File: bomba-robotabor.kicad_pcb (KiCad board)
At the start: 2 copper layers, 46 parts, among them U1 74HC03, U2 74HCT08, U3 L4904

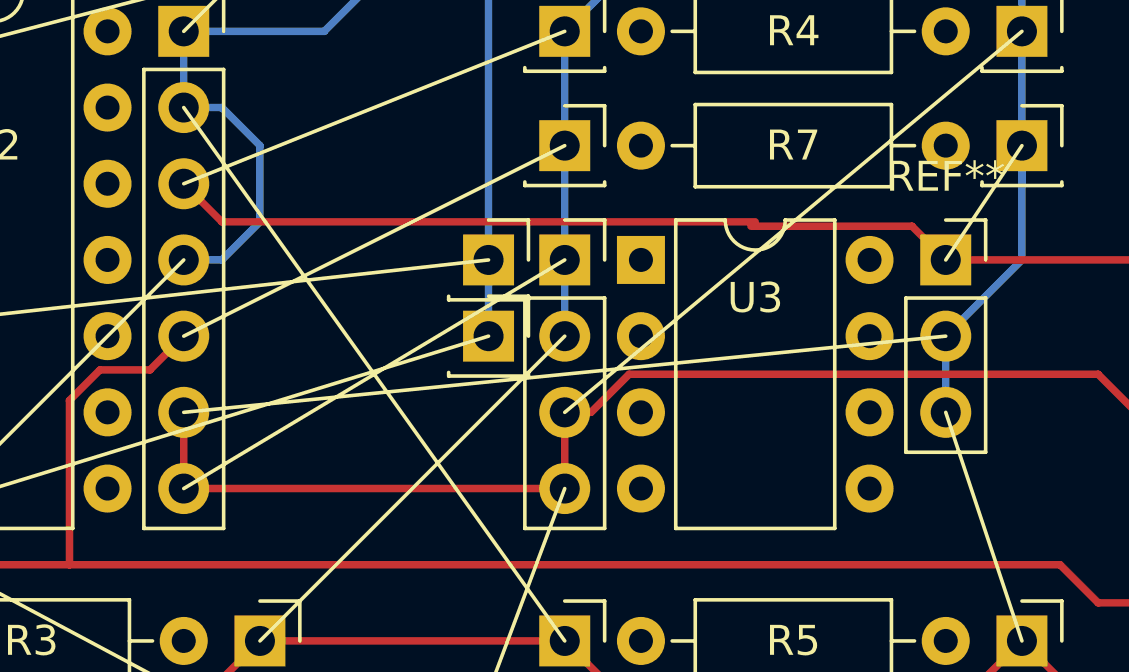
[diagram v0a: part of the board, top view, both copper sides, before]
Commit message: fixed mistake
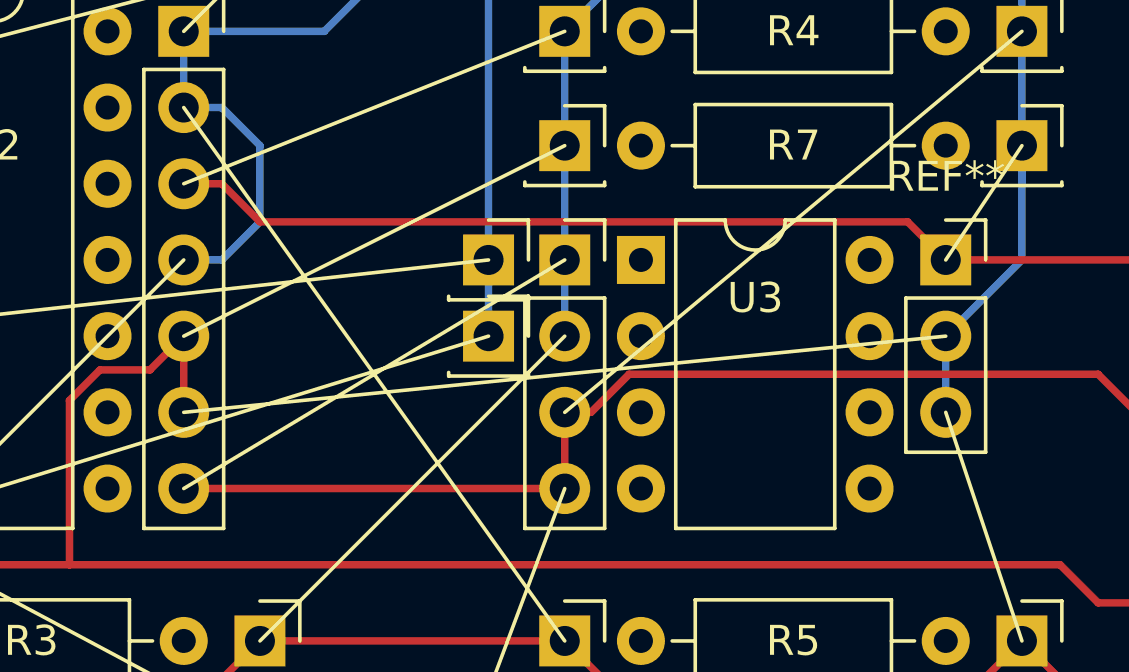
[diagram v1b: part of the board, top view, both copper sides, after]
